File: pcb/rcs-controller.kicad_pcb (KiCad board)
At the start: 2 copper layers, 45.6 x 73 mm, 100 parts, among them J1 00222-32051, J10 0022-232021, J2 0022-232021, J3 0022-232041, J4 Screw_Terminal_4_P3.50mm, J5 USB_C_Receptacle_USB2.0_14P, J6 Conn_01x03, J8 00222-32051, Q1 SI7465DP-T1-E3, Q2 SI7465DP-T1-E3, Q3 SI7465DP-T1-E3, Q4 PMV45EN2, Q5 PMV45EN2, SW1 SW_Push, U1 LSM6DSOX, U2 MP26123DR-LF-Z, U3 TPS63070, U4 ESP32-S3-WROOM-1

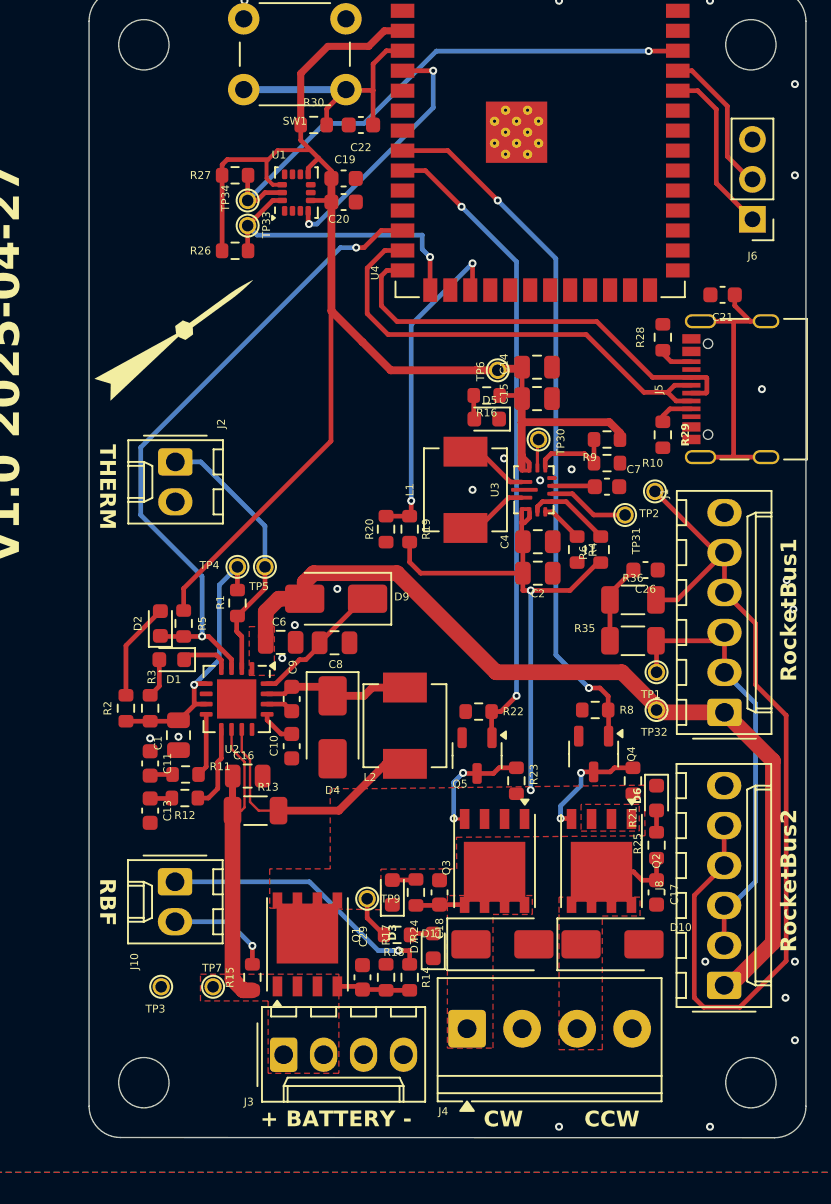
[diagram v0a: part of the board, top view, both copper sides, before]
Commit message: Silkscreen clean up
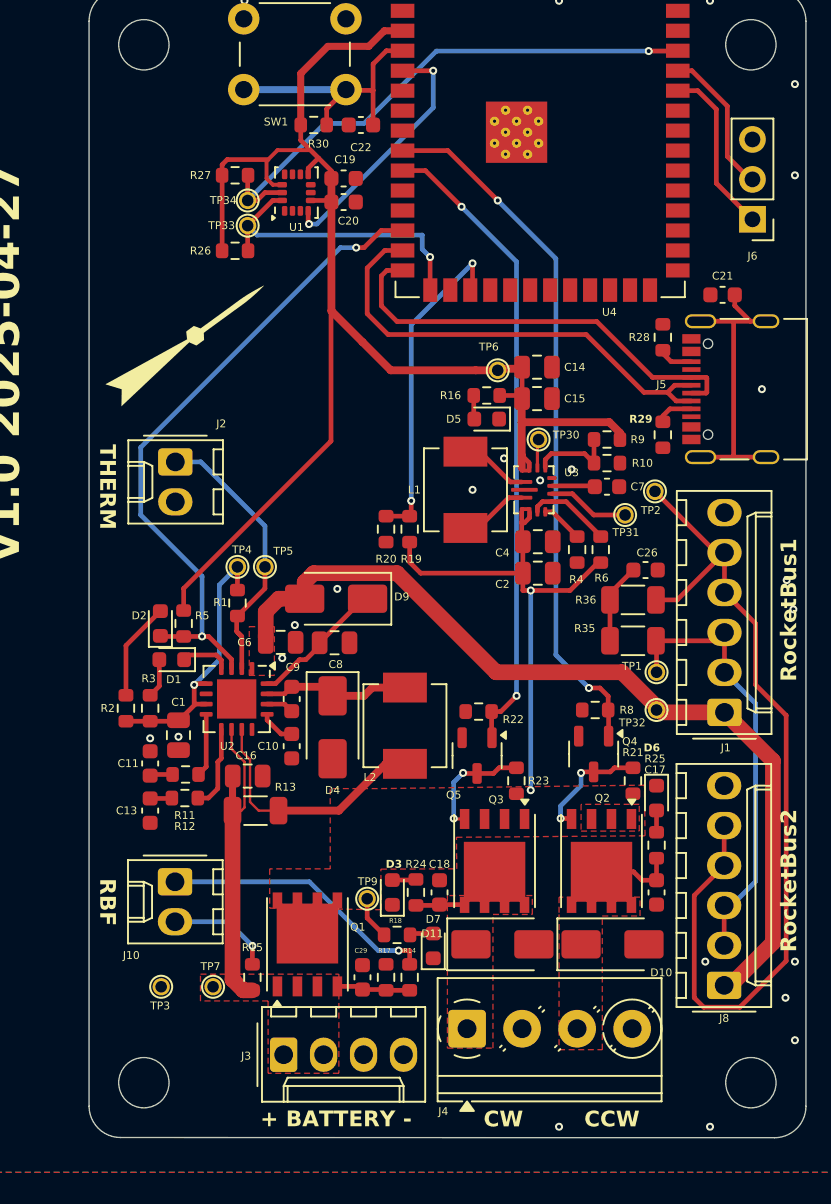
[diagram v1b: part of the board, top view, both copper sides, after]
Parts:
- moved LOGO1 0.78 mm to (106.5, 100.5)
